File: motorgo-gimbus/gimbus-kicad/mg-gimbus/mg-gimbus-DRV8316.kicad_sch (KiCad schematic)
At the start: 14 parts, among them U12 DRV8316CRRGFR

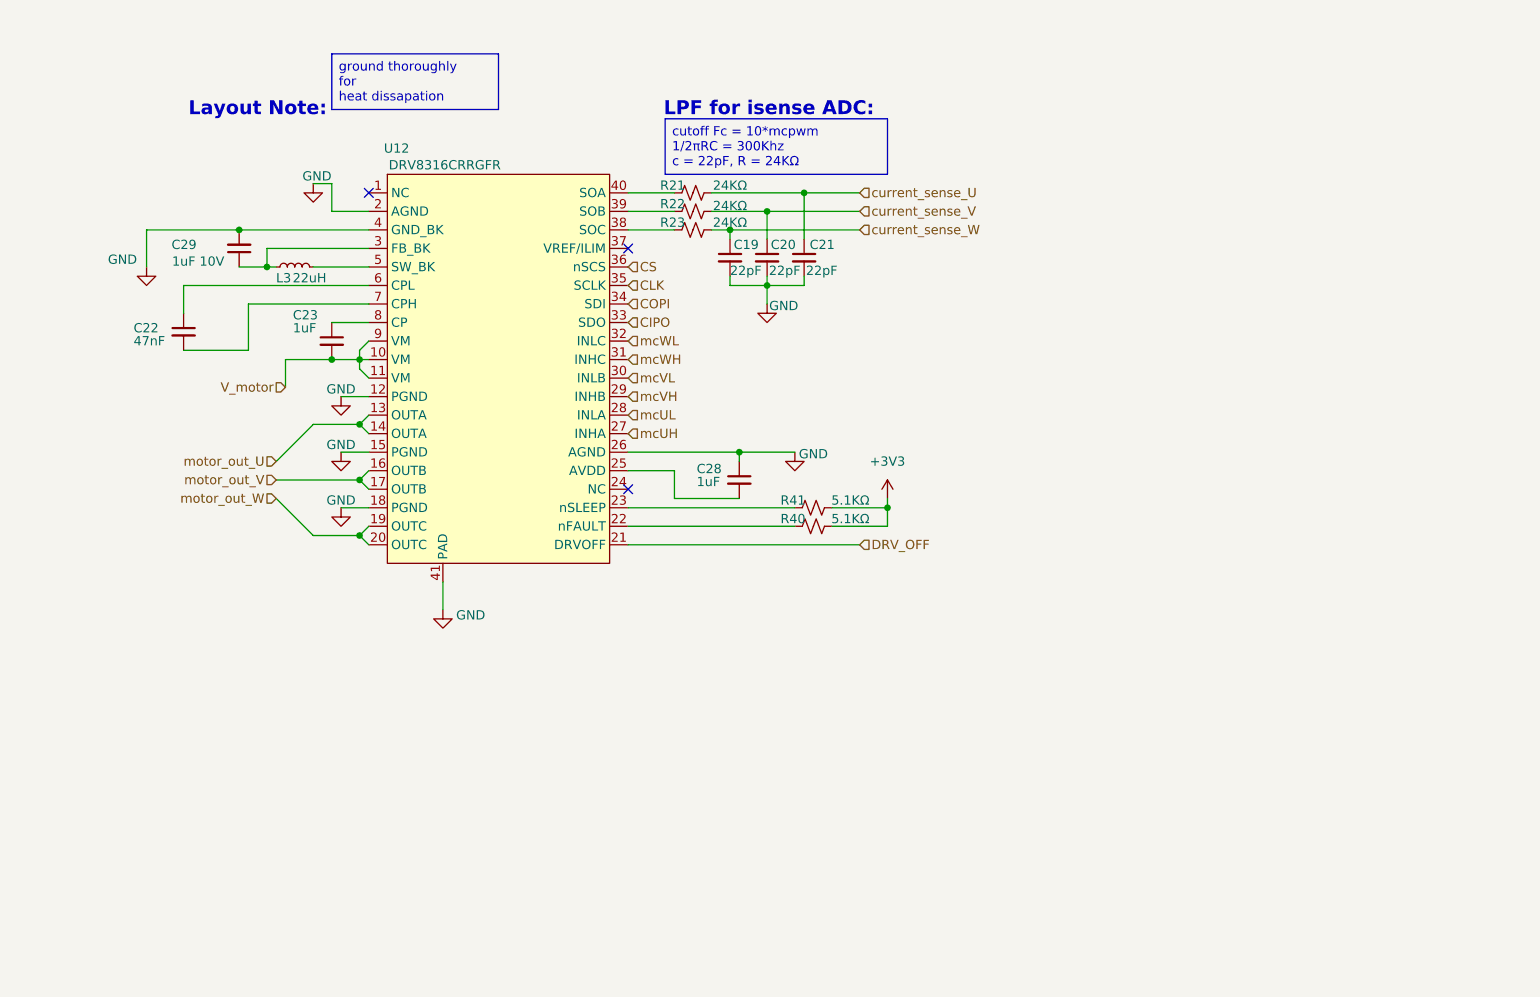
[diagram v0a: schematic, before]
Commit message: incremental layout progress
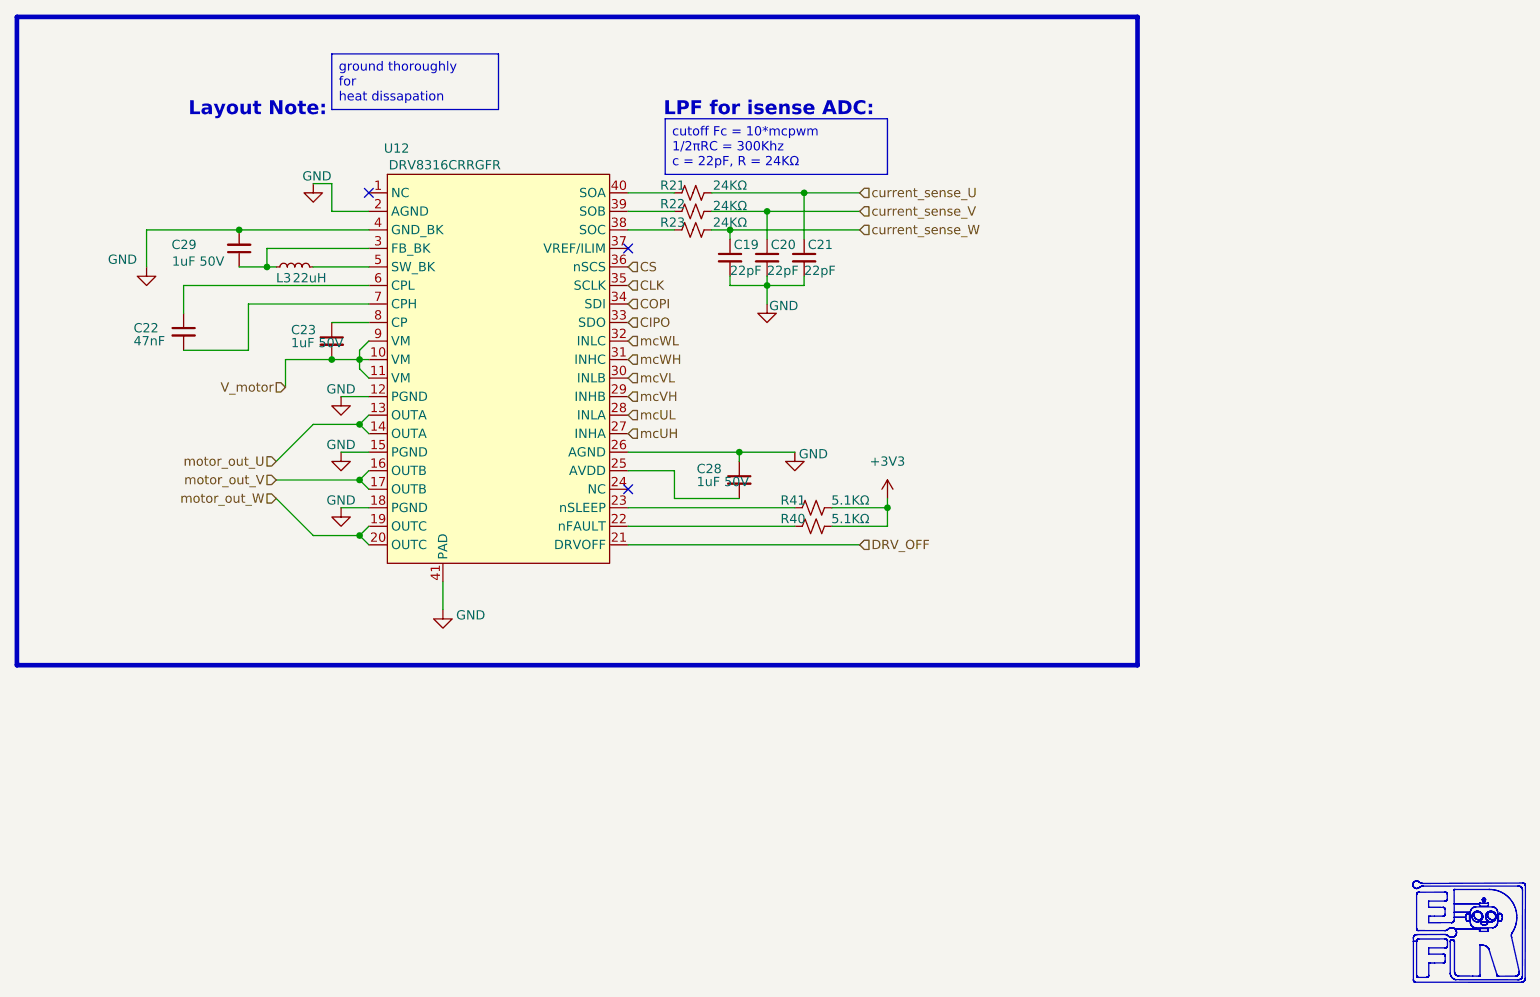
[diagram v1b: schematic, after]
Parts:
- C19, C20, C21: footprint (none) -> Capacitor_SMD:C_0402_1005Metric; LCSC Part (none) -> C76960
- C22: footprint (none) -> Capacitor_SMD:C_0402_1005Metric; LCSC Part (none) -> C82219
- C23, C28: value 1uF -> 1uF 50V; footprint (none) -> Capacitor_SMD:C_0805_2012Metric; LCSC Part (none) -> C28323
- C29: value 1uF 10V -> 1uF 50V; footprint (none) -> Capacitor_SMD:C_0805_2012Metric; LCSC Part (none) -> C28323
- L3: footprint (none) -> Inductor_SMD:L_0603_1608Metric; LCSC Part (none) -> C383393
- R21, R22, R23: footprint (none) -> Resistor_SMD:R_0402_1005Metric; LCSC Part (none) -> C25769
- R40, R41: footprint (none) -> Resistor_SMD:R_0402_1005Metric; LCSC Part (none) -> C25905
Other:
- company: (none) -> MotorGo LLC
- title: (none) -> MotorGo Gimbus
